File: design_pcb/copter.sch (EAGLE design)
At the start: 57 parts, among them U1 ATMEGA328P-AU, U10 INA169, U2 ITG-3200, U3 ADXL345, U5 HC_05, U6 IRF9362PBF, U7 IRF9362PBF, U8 HMC5883LSMD, U9 3.3V, Y1 8MHZ

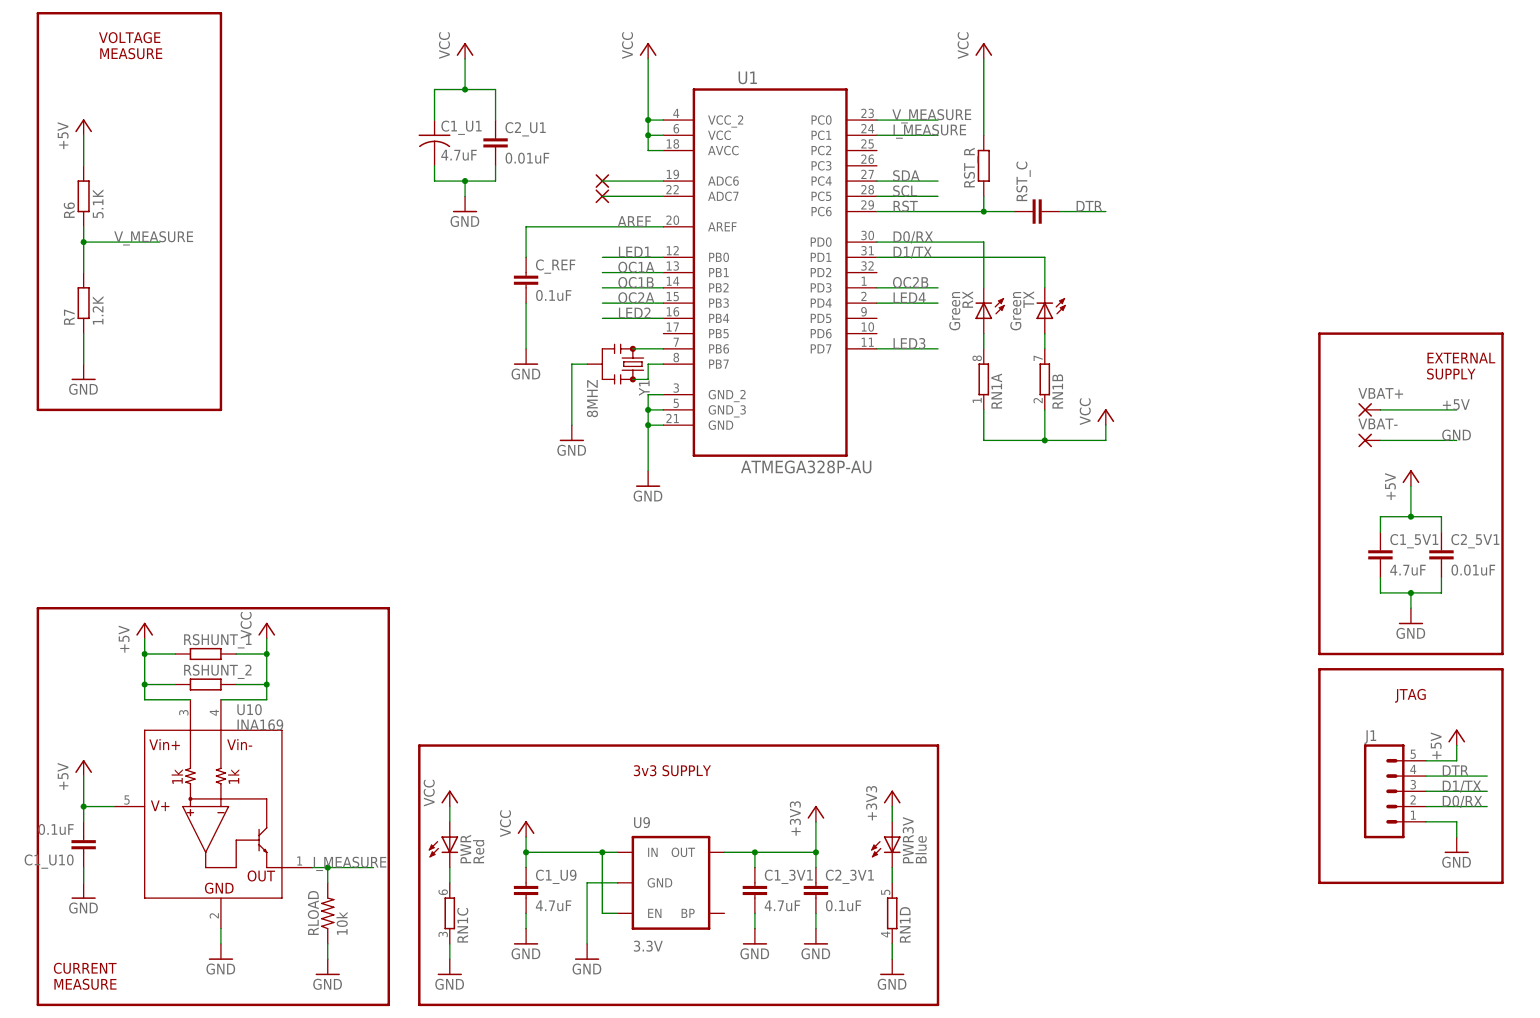
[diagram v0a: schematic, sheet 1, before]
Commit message: Update schematic and PCB
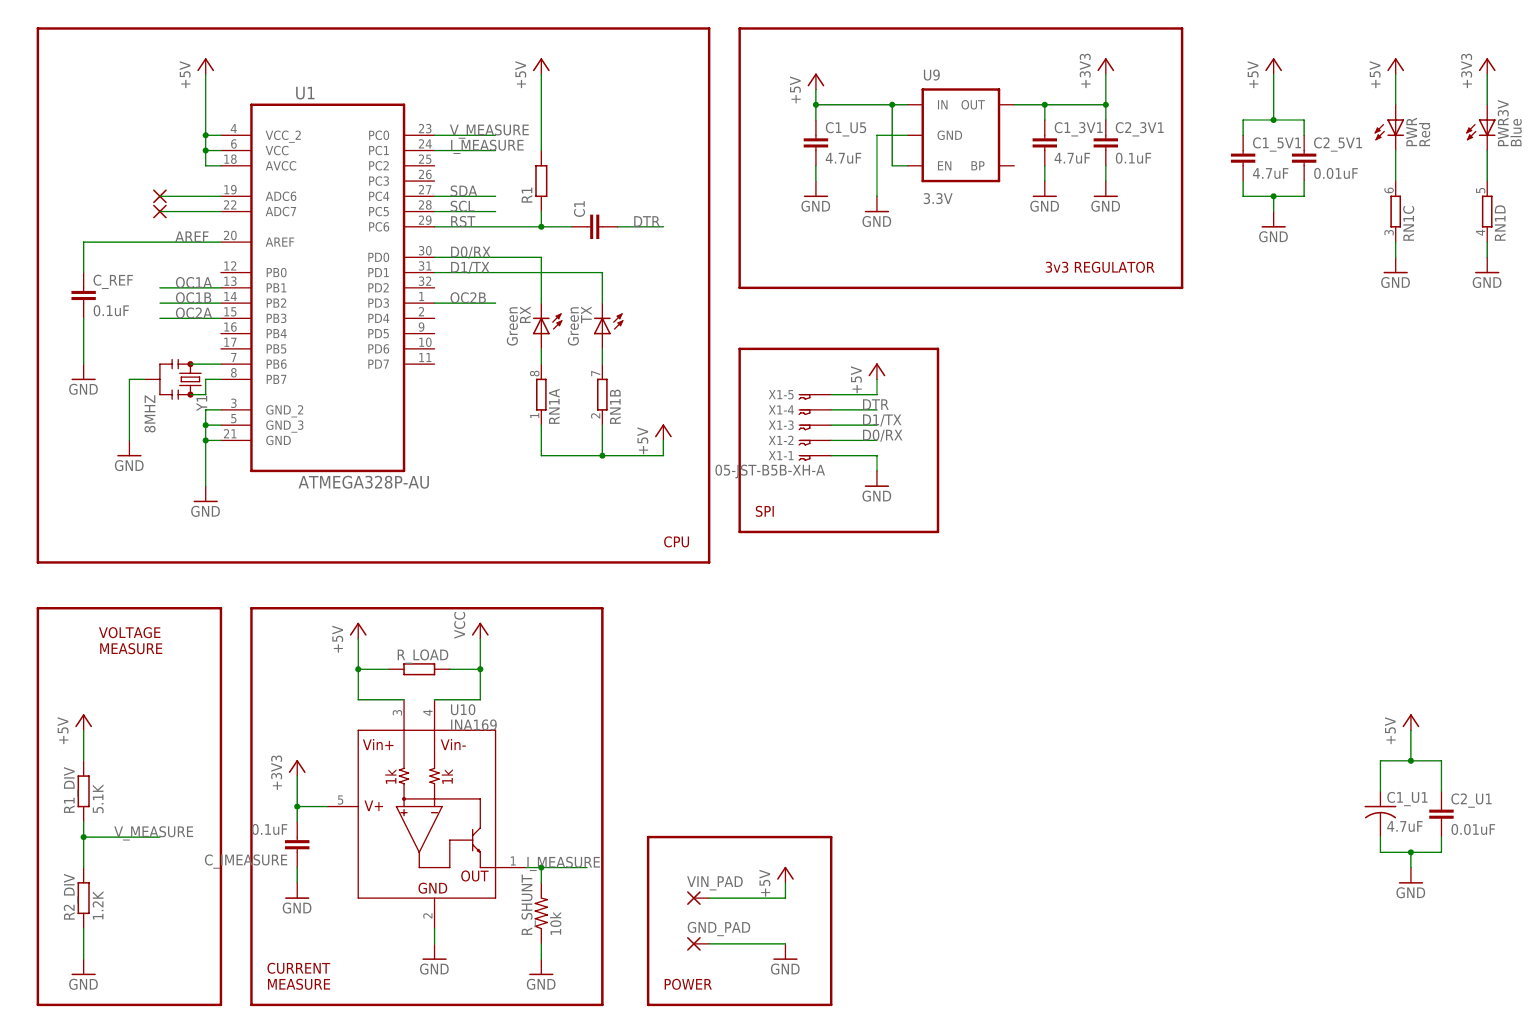
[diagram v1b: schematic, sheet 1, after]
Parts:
- removed C1_U10: 0.1uF, SparkFun-Passives:CAP0603-CAP
- removed C1_U9: 4.7uF, SparkFun:CAP0402-CAP
- removed J1: (no value), SparkFun-Connectors:M05PTH
- removed LED1, LED2, LED3, LED4: (no value), led:LED3MM
- removed R6: 5.1K, resistor:R-EU_R0402
- removed R7: 1.2K, resistor:R-EU_R0402
- removed RLOAD: 10k, SparkFun-Resistors:RESISTOR0603
- removed RSHUNT_1, RSHUNT_2: (no value), resistor:R-EU_0309/10
- removed RST_C: (no value), rcl:C-EUC0402
- removed RST_R: (no value), rcl:R-EU_R0402
- removed VBAT+, VBAT-: (no value), wirepad:1,6/0,8
- added C1: (no value), rcl:C-EUC0402
- added C1_U5: 4.7uF, SparkFun:CAP0402-CAP
- added C_IMEASURE: 0.1uF, SparkFun-Passives:CAP0603-CAP
- added GND_PAD, VIN_PAD: (no value), wirepad:1,6/0,8
- added R1: (no value), rcl:R-EU_R0402
- added R1_DIV: 5.1K, resistor:R-EU_R0402
- added R2_DIV: 1.2K, resistor:R-EU_R0402
- added R_LOAD: (no value), resistor:R-EU_0309/10
- added R_SHUNT: 10k, SparkFun-Resistors:RESISTOR0603
- added X1: 05-JST-B5B-XH-A, bt_con-jst-xh:05-JST-B5B-XH-A
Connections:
- net MTR3 renamed N$31
- net MTR4 renamed N$15
- removed net LED1: LED3.A, U1.PB0
- removed net LED2: LED4.A, U1.PB4
- removed net LED3: LED1.A, U1.PD7
- removed net LED4: LED2.A, U1.PD4
- net +3V3: now also C_IMEASURE.2, U10.V+
- net +5V: now also C1_U1.1, C1_U5.1, C2_U1.1, PWR.A, R1.2, R1_DIV.2, RN1A.1, RN1B.1, R_LOAD.1, U1.AVCC, U1.VCC, U1.VCC_2, U9.EN, U9.IN, VIN_PAD.P, X1-5.1; no longer C1_U10.2, J1.5, R6.2, RSHUNT_1.1, RSHUNT_2.1, U10.V+, VBAT+.P
- net D0/RX: now also X1-2.1; no longer J1.2
- net D1/TX: now also X1-3.1; no longer J1.3
- net DTR: now also C1.2, X1-4.1; no longer J1.4, RST_C.2
- net GND: now also C1_U5.2, C_IMEASURE.1, GND_PAD.P, R2_DIV.1, R_SHUNT.1, X1-1.1; no longer C1_U10.1, C1_U9.2, J1.1, LED1.C, LED2.C, LED3.C, LED4.C, R7.1, RLOAD.1, VBAT-.P
- net I_MEASURE: now also R_SHUNT.2; no longer RLOAD.2
- net RST: now also C1.1, R1.1; no longer RST_C.1, RST_R.1
- net VCC: now also R_LOAD.2; no longer C1_U1.1, C1_U9.1, C2_U1.1, PWR.A, RN1A.1, RN1B.1, RSHUNT_1.2, RSHUNT_2.2, RST_R.2, U1.AVCC, U1.VCC, U1.VCC_2, U9.EN, U9.IN
- net V_MEASURE: now also R1_DIV.1, R2_DIV.2; no longer R6.1, R7.2
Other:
- note added: "3v3 REGULATOR"
- note added: "CPU"
- note added: "POWER"
- note added: "SPI"
- note removed: "3v3 SUPPLY"
- note removed: "EXTERNAL SUPPLY"
- note removed: "JTAG"
- moved on the sheet: C1_3V1, C1_5V1, C1_U1, C2_3V1, C2_5V1, C2_U1, C_REF, MTR1_1, MTR1_2, MTR2_1, MTR2_2, MTR3_1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
